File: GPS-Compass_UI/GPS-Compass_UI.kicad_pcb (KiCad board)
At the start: 2 copper layers, 15 x 75 mm, 24 parts, among them J4 Conn_01x10_Socket, SW1 SPDT, SW3 RESET, SW4 EXT, SW5 RESET, SW6 EXT, SW7 EXT, SW8 EXT

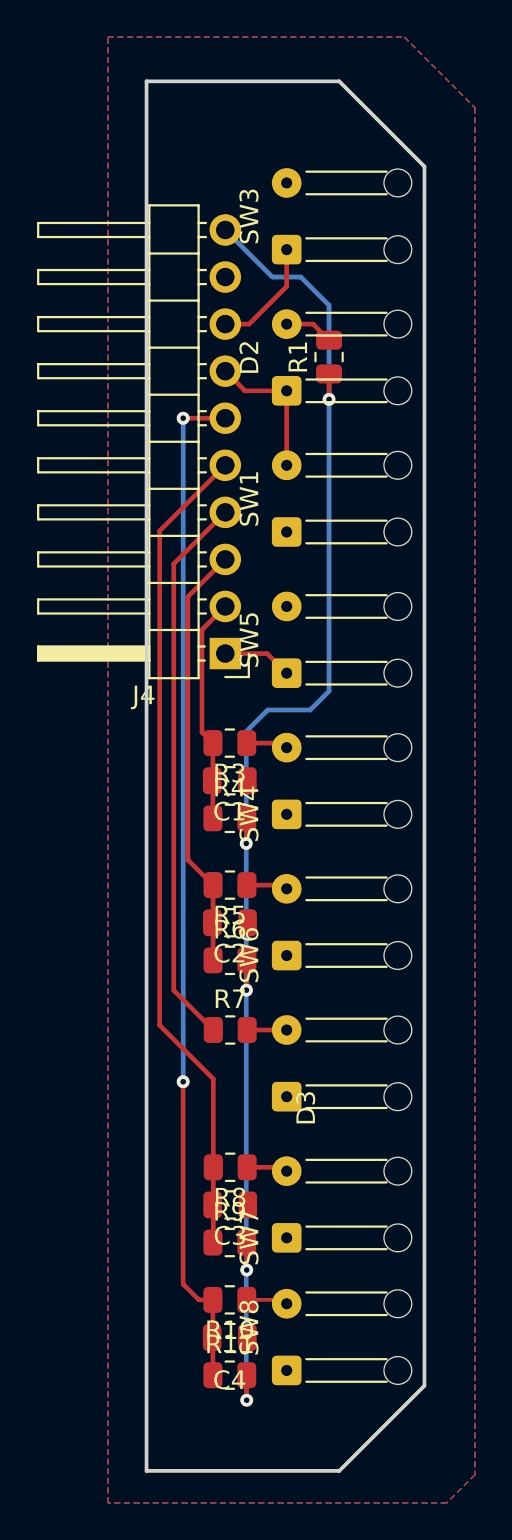
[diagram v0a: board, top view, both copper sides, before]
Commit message: UI board updates
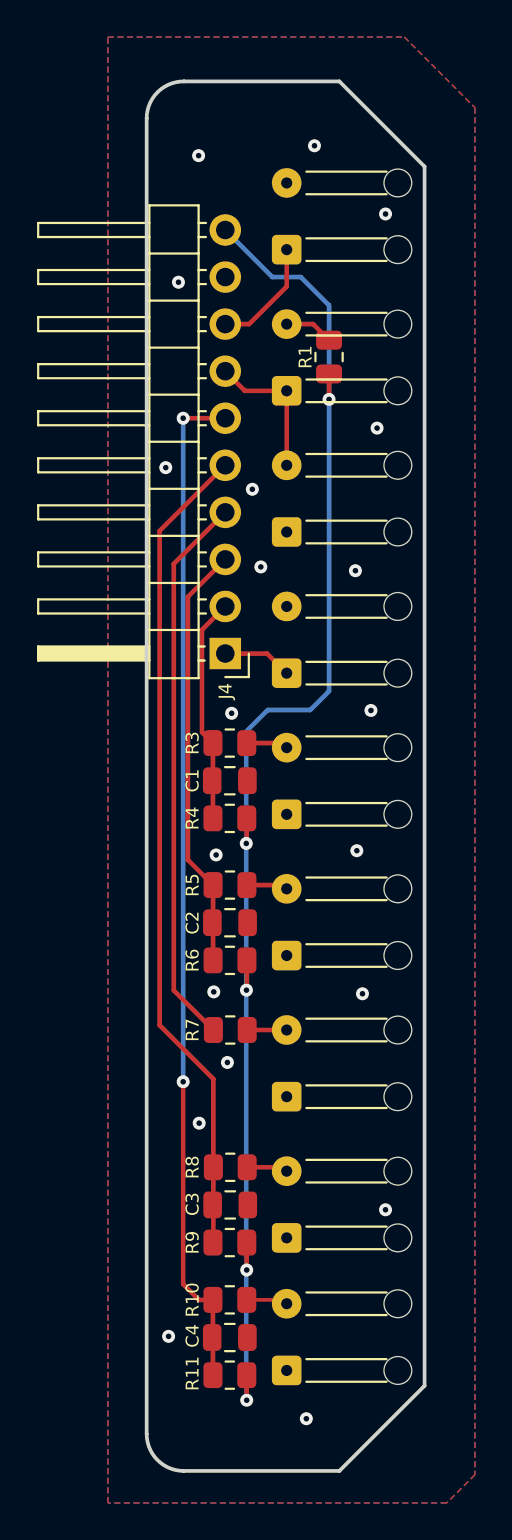
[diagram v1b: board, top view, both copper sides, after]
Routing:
- net GND: vias 0 -> 20
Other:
- outline, holes or cut-outs redrawn

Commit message: updates on different boards
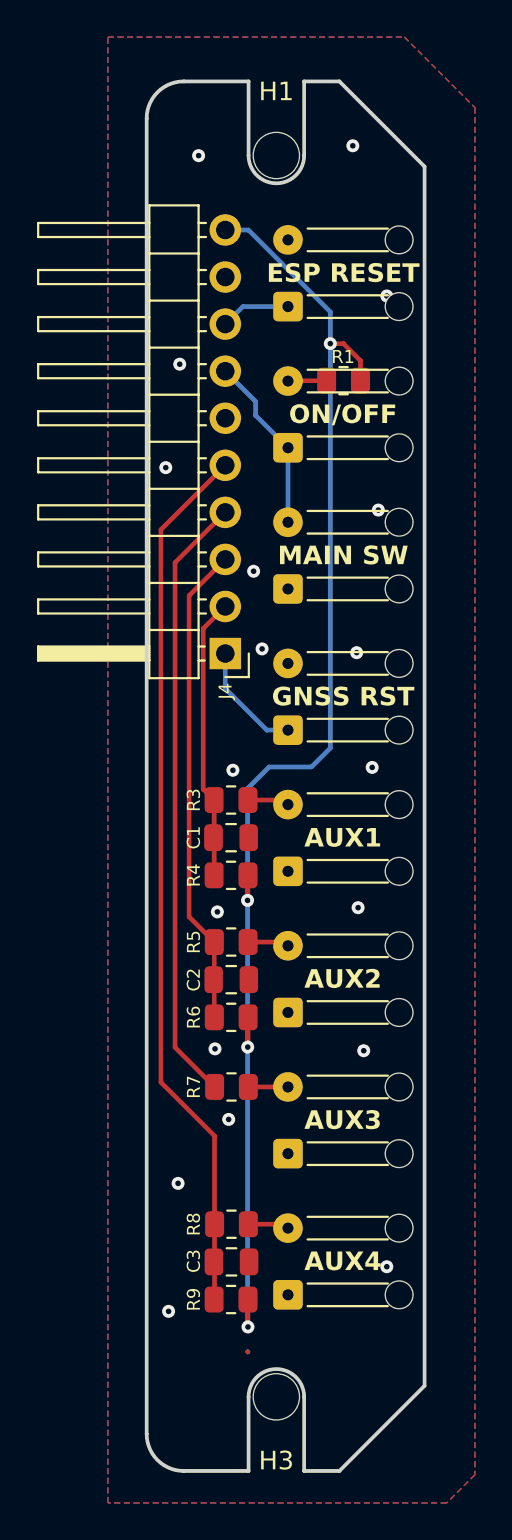
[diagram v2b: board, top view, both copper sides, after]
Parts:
- removed C4: 100nF, Capacitor_SMD:C_0805_2012Metric
- removed R10: 1k, Resistor_SMD:R_0805_2012Metric
- removed R11: 10k, Resistor_SMD:R_0805_2012Metric
- removed SW8: EXT, Connector_Wire:SolderWire-0.1sqmm_1x02_P3.6mm_D0.4mm_OD1mm_Relief
- added H1: M2.5, MountingHole:MountingHole_2.5mm, F.Cu at (122.1, 66.8)
- added H3: M2.5, MountingHole:MountingHole_2.5mm, F.Cu at (122.1, 133.8)
- moved C1 3.07 mm to (119.7, 103.7)
- moved C2 3.07 mm to (119.7, 111.3)
- moved C3 3.07 mm to (119.7, 126.6)
- moved D2 3.07 mm to (122.8, 82.6)
- moved D3 3.07 mm to (122.8, 120.7)
- moved R3 3.07 mm to (119.7, 101.6)
- moved R4 3.07 mm to (119.7, 105.7)
- moved R5 3.07 mm to (119.7, 109.3)
- moved R6 3.07 mm to (119.7, 113.4)
- moved R7 3.07 mm to (119.7, 117.1)
- moved R8 3.07 mm to (119.7, 124.5)
- moved R9 3.07 mm to (119.7, 128.6)
- moved SW1 3.07 mm to (122.8, 90.2)
- moved SW3 3.07 mm to (122.8, 75.0)
- moved SW4 3.07 mm to (122.8, 105.5)
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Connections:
- J4 pad 6: /DBNCD_3 -> GND
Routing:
- net /DBNCD_3: track 55.0 -> 0.00 mm, vias 2 -> 0
- net +3V3: track 76.8 -> 73.0 mm, vias 5 -> 4
- net /DBNCD_1: track 23.0 -> 26.1 mm
- net /DBNCD_0: track 12.2 -> 15.2 mm
- net /LED_EXT: track 30.0 -> 33.0 mm
- net /DBNCD_2: track 44.6 -> 47.7 mm
- net /GNSS_RST: track 3.75 -> 6.20 mm
- net /DB_3: track 2.43 -> 0.00 mm
- net /EN: track 6.14 -> 3.77 mm
- net /MSW_ON: track 7.77 -> 9.56 mm
- net Net-(D2-A): track 2.64 -> 2.10 mm
- net GND: vias 20 -> 19
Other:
- outline, holes or cut-outs redrawn
- board text added: "AUX1"
- board text added: "AUX2"
- board text added: "AUX3"
- board text added: "AUX4"
- board text added: "ESP RESET"
- board text added: "GNSS RST"
- board text added: "MAIN SW"
- board text added: "ON/OFF"
